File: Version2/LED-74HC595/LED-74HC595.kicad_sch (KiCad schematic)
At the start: 11 parts, among them J1 Conn_02x19_Odd_Even, J2 Conn_01x08_Pin, J3 Conn_01x10_Pin, SW1 SW_Push, U2 74HC595, U3 74HC595, U4 74HC595

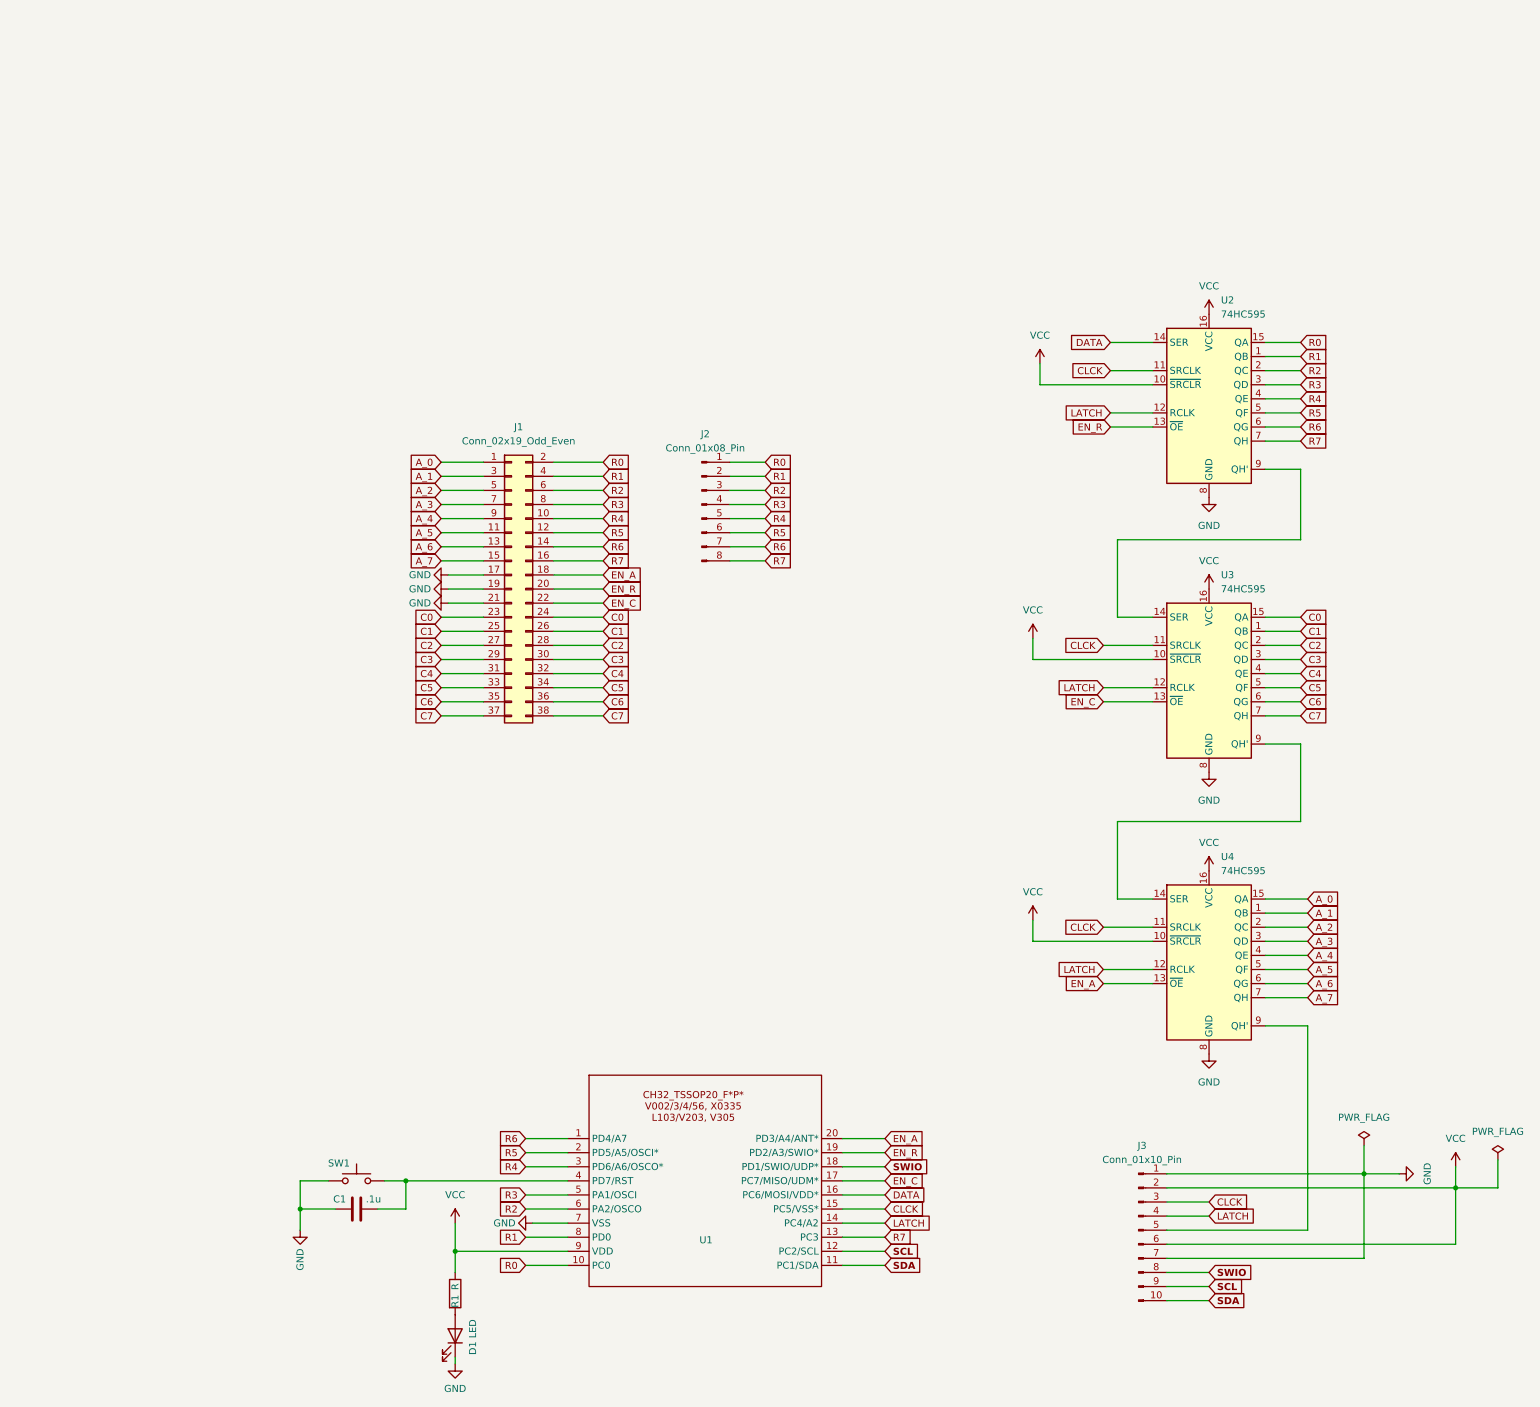
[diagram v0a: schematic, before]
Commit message: update.
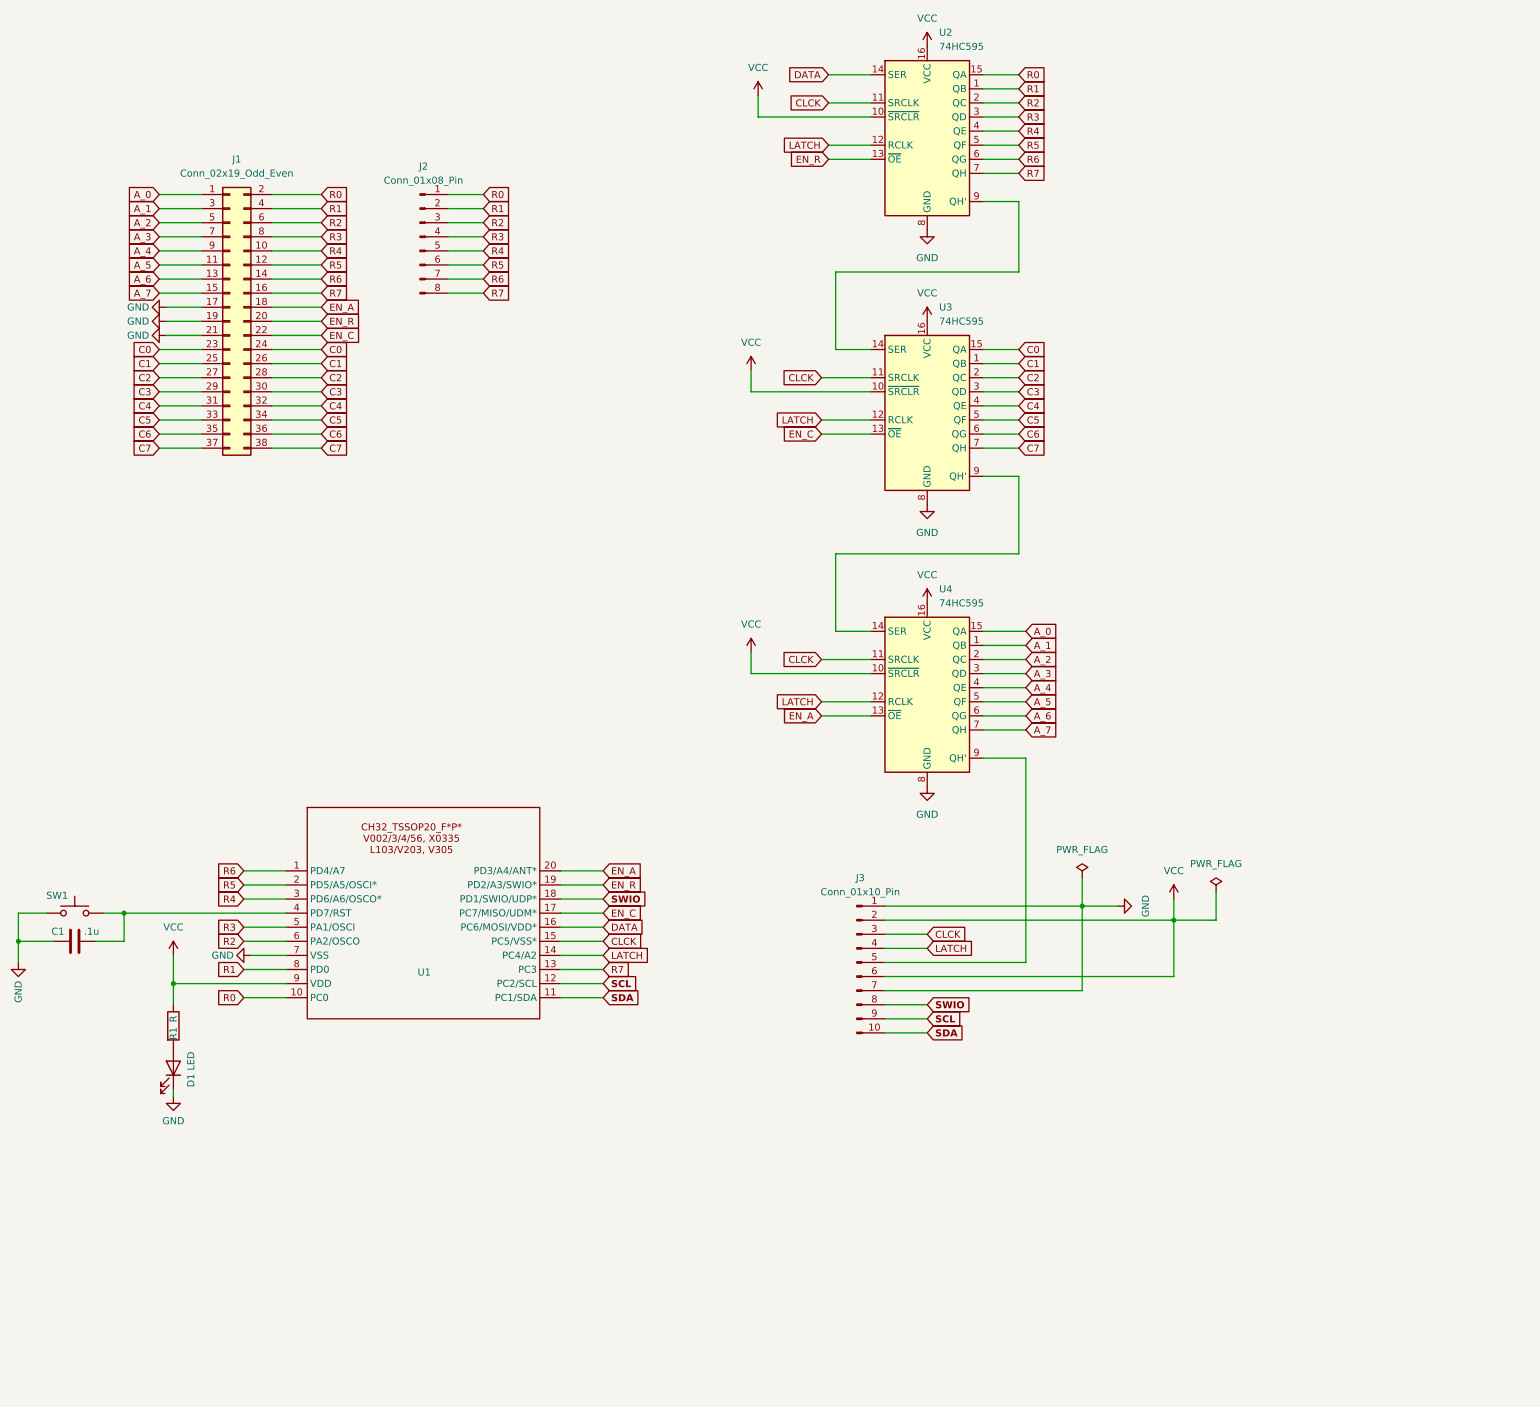
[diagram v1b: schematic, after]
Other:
- moved on the sheet: C1, D1, J1, J2, J3, R1, SW1, U1, U2, U3, U4
